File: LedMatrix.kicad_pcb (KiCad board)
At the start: 2 copper layers, 32 x 32 mm, 30 parts, among them IC1 ATMEGA328P-A, P1 FTDI, P2 SYNC_OUT, P3 ICSP, SW1 SW_PUSH, SW2 SWITCH_INV, U1 74HC238, U2 TD62083AFNG, U3 MCP1700-3302, U4 PNJ4K01F, U5 ADXL345, X1 8Mhz

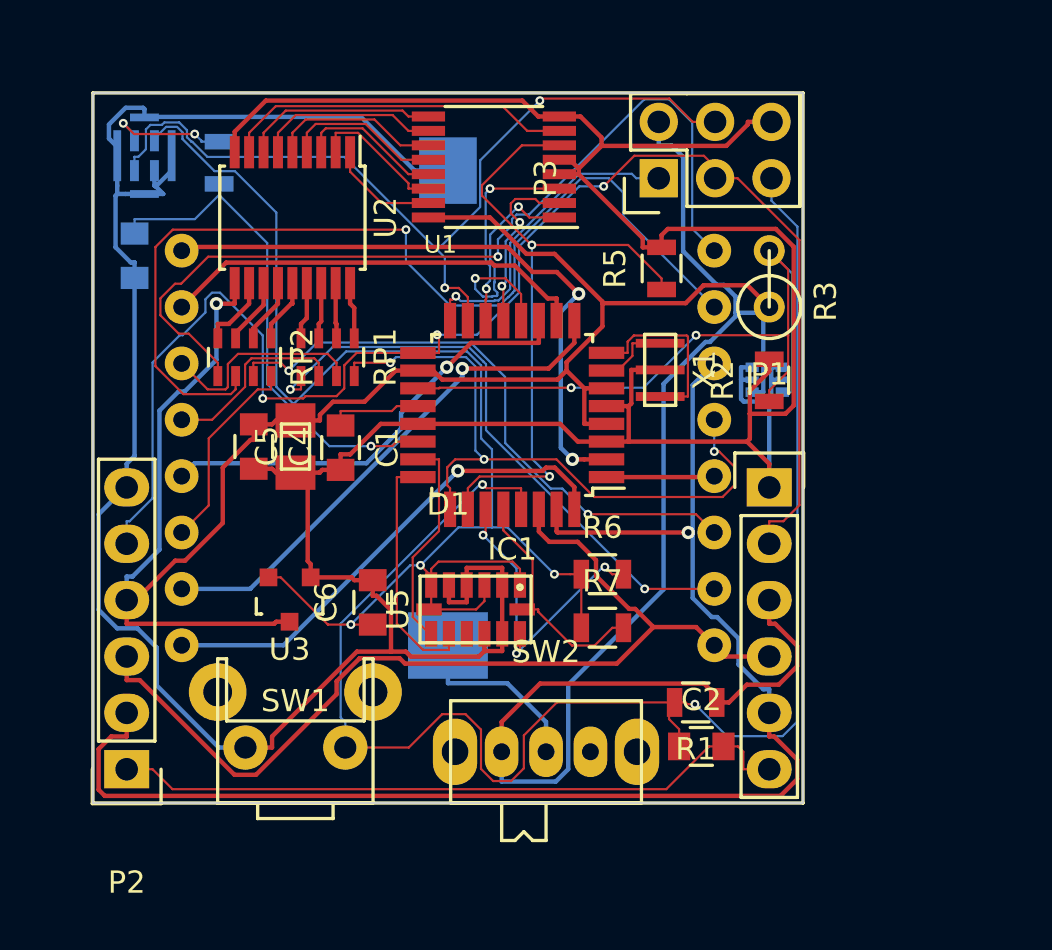
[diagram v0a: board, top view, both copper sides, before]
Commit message: Brightness code
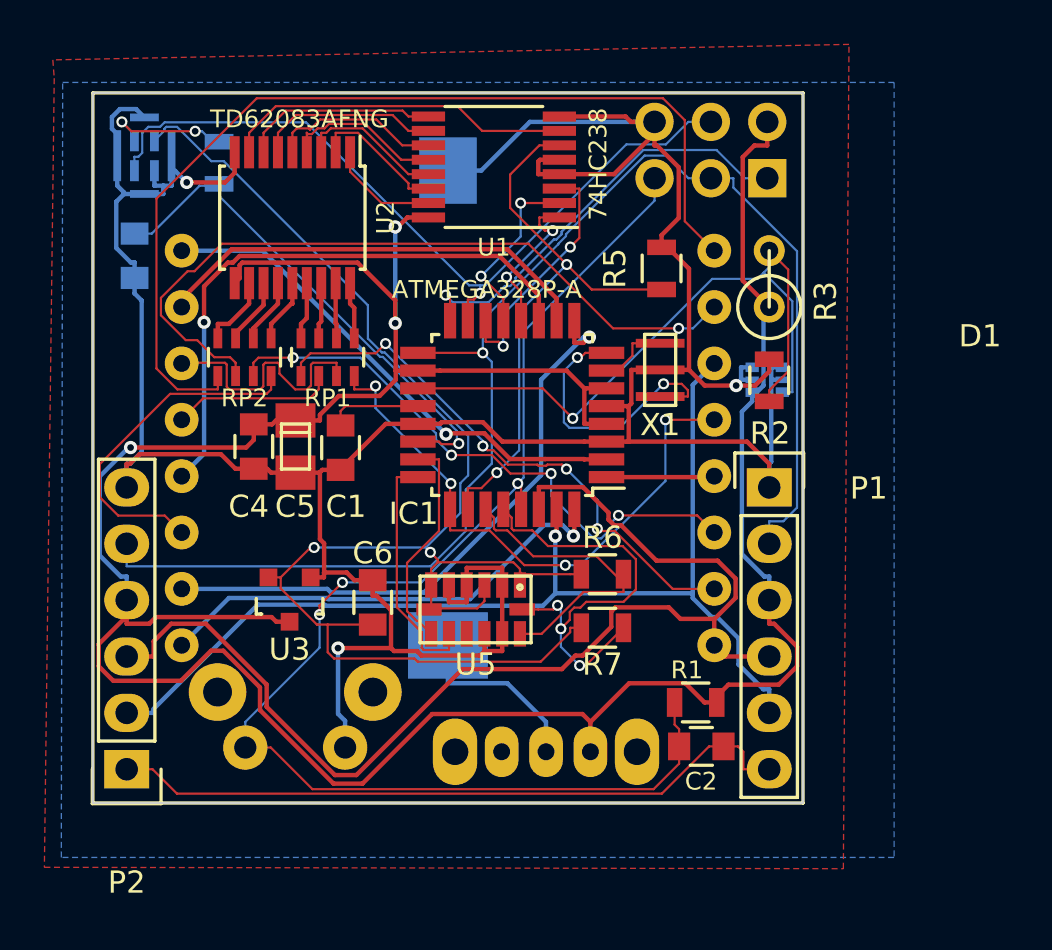
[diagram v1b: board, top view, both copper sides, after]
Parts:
- P3, SW1, SW2: moved to B.Cu
- moved P3 4.89 mm to (64.4, 37.8)
- turned SW1 to 180 degrees
- turned SW2 to 180 degrees
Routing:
- net GND: track 188.6 -> 149.9 mm, vias 0 -> 3
- net /ROW2: track 65.0 -> 49.6 mm
- net VCC: track 143.3 -> 132.1 mm, vias 1 -> 3
- net Net-(D1-Pad15): track 44.6 -> 33.6 mm
- net /RESET: track 71.1 -> 60.2 mm, vias 2 -> 3
- net /SCL: track 10.7 -> 20.4 mm, vias 0 -> 3
- net /ROW1: track 44.0 -> 52.5 mm
- net /ROW8: track 20.0 -> 26.5 mm
- net Net-(D1-Pad6): track 9.07 -> 15.5 mm
- net /ROW5: track 28.4 -> 23.1 mm, vias 2 -> 1
- net /MISO: track 14.2 -> 19.4 mm
- net Net-(IC1-Pad12): track 11.9 -> 7.14 mm
- net /LOWSIDE_EN: track 30.5 -> 25.8 mm
- net Net-(IC1-Pad8): track 8.26 -> 12.7 mm, vias 0 -> 2
- net Net-(D1-Pad16): track 39.8 -> 43.9 mm, vias 1 -> 0
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- added copper zone on B.Cu, net GND
- added copper zone on F.Cu, net GND
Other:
- net class SIGNAL: via_dia 0.4 -> 0.5; via_drill 0.2 -> 0.3
- board text added: "DotDotLab"
- board text added: "EdwardRF Mika Lin"

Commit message: Add francis and northy mods
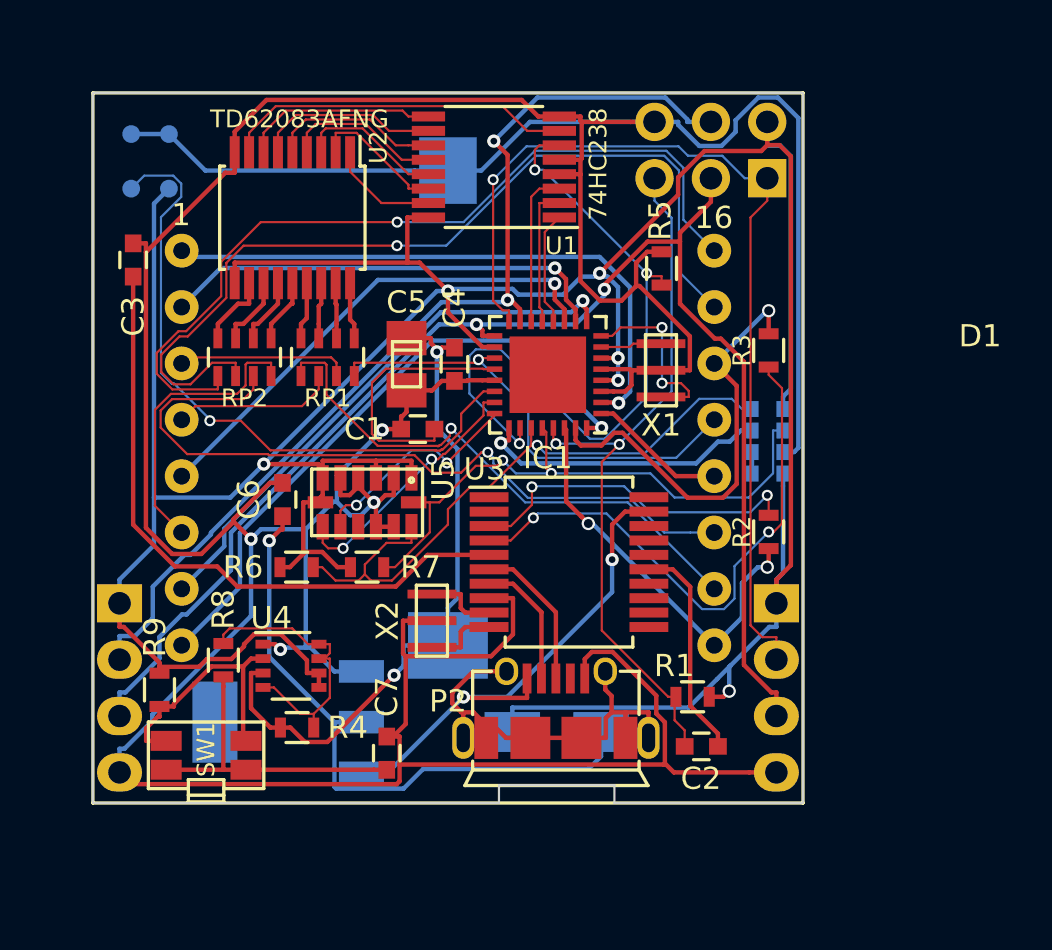
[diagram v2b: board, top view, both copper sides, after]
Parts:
- removed S1: MP34DT01, MP34DT01:MP34DT01
- removed SW2: SWITCH_INV, 1P2T:1P2T_SideSwitch
- added C7: 1uf, Capacitors_SMD:C_0603, F.Cu at (47.2, 63.8)
- added D2: D_Schottky, Diodes_SMD:SMA_Standard, B.Cu at (54.9, 62.8)
- added M1: 3729Mic, 3729Mic:3729Mic, B.Cu at (36.6, 37.1)
- added P0: CONN_01X04, Pin_Headers:Pin_Header_Straight_1x04, B.Cu at (64.8, 57.0)
- added R8: 100k, Resistors_SMD:R_0603, F.Cu at (39.9, 59.6)
- added R9: 10k, Resistors_SMD:R_0603, F.Cu at (37.0, 60.9)
- added U6: APDS-9900, ADPS-9900:ADPS-9900, B.Cu at (64.4, 49.7)
- added U7: AP1117D30, TO_SOT_Packages_SMD:SOT-223, B.Cu at (42.8, 62.4)
- added X2: 12Mhz, CSTCE8M:CSTCE8M00G52, F.Cu at (49.3, 57.8)
- C1, C2, C4, C6: footprint Capacitors_SMD:C_0805 -> Capacitors_SMD:C_0603
- C3: value 10nf -> 0.1uf; footprint Capacitors_SMD:C_0805 -> Capacitors_SMD:C_0603; moved to F.Cu
- IC1: footprint Housings_QFP:TQFP-32_7x7mm_Pitch0.8mm -> Housings_DFN_QFN:QFN-32-1EP_5x5mm_Pitch0.5mm
- P1: value FTDI -> CONN_01X04; footprint Pin_Headers:Pin_Header_Straight_1x06 -> Pin_Headers:Pin_Header_Straight_1x04; moved to B.Cu
- P2: value SYNC_OUT -> USB_OTG; footprint Pin_Headers:Pin_Header_Straight_1x06 -> Molex475890001:47589-0001
- R1, R2, R5, R6, R7: footprint Resistors_SMD:R_0805 -> Resistors_SMD:R_0603
- R3: value Photores -> 100k; footprint Discret:R1 -> Resistors_SMD:R_0603
- R4: footprint Resistors_SMD:R_0805 -> Resistors_SMD:R_0603; moved to F.Cu
- SW1: footprint SideButton:SidePushButton -> SKSCLCE010:SKSCLCE010; moved to F.Cu
- U3: value MCP1700-3302 -> CH340T; footprint Housings_SOT-23_SOT-143_TSOT-6:SOT-23 -> Housings_SSOP:SSOP-20_5.3x7.2mm_Pitch0.65mm
- U4: value PNJ4K01F -> TPCP8405; footprint pnj4k01f:KPTFTN6K0001 -> ps_8:PS-8; moved to F.Cu
- moved P1 29.7 mm to (35.2, 57.0), turned to 180 degrees
- moved R4 25.7 mm to (43.2, 62.6), turned to 0 degrees
- moved U4 25.0 mm to (42.9, 59.8)
- moved P2 19.4 mm to (54.9, 63.1), turned to 0 degrees
- moved R6 13.8 mm to (43.2, 55.4)
- moved U3 12.7 mm to (55.5, 55.1), turned to 0 degrees
- moved R7 11.0 mm to (46.4, 55.4)
- moved C4 9.77 mm to (50.3, 46.2)
- moved U5 6.87 mm to (46.4, 52.5)
- moved R2 6.83 mm to (64.5, 53.8)
- moved C5 6.23 mm to (48.1, 46.2)
- moved C6 6.16 mm to (42.5, 52.3)
- moved SW1 4.03 mm to (39.1, 63.9), turned to 0 degrees
- moved C1 3.58 mm to (48.6, 49.1), turned to 180 degrees
- moved R3 3.23 mm to (64.5, 45.6), turned to 270 degrees
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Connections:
- C2 pad 2: /DTR -> Net-(C2-Pad2)
- C3 pad 1: /AUDIO_IN -> GND
- C3 pad 2: GND -> Net-(C3-Pad2)
- C4 pad 1: VCC -> Net-(BT1-Pad1)
- C5 pad 1: VCC -> Net-(BT1-Pad1)
- C6 pad 1: /3v3 -> Net-(C6-Pad1)
- IC1 pad 15: /AUDIO_CLK -> /MOSI
- IC1 pad 17: /RTS -> /SCK
- IC1 pad 19: /LIGHT_SENSE -> /LED_SENSE
- IC1 pad 25: /LED_SENSE -> /LIGHT_INT
- P1 pad 1: GND -> VCC
- P1 pad 2: /RTS -> /MOSI
- P1 pad 3: VCC -> /SCK
- P1 pad 4: /ROW1 -> GND
- P2 pad 1: /DTR -> /5V
- P2 pad 2: /ROW2 -> /D-
- P2 pad 3: /ROW1 -> /D+
- P2 pad 4: VCC -> (no net)
- P2 pad 5: /RTS -> GND
- P2 pad 6: GND -> Net-(P2-Pad6)
- P3 pad 3: /RTS -> /SCK
- P3 pad 4: /AUDIO_CLK -> /MOSI
- R2 pad 1: /LIGHT_SENSE -> /ROW1
- R2 pad 2: GND -> Net-(R2-Pad2)
- R3 pad 1: VCC -> /ROW2
- R3 pad 2: /LIGHT_SENSE -> Net-(R3-Pad2)
- R4 pad 1: /AUDIO_IN -> Net-(BT1-Pad1)
- R6 pad 1: /3v3 -> VCC
- R7 pad 1: /3v3 -> VCC
- SW1 pad 1: GND -> Net-(C7-Pad1)
- SW1 pad 2: /RESET -> Net-(R9-Pad2)
- U3 pad 1: GND -> (no net)
- U3 pad 2: /3v3 -> (no net)
- U3 pad 3: VCC -> Net-(R2-Pad2)
- U4 pad 1: VCC -> GND
- U4 pad 2: GND -> Net-(R9-Pad2)
- U4 pad 3: GND -> Net-(BT1-Pad1)
- U4 pad 4: GND -> Net-(R4-Pad2)
- U4 pad 5: GND -> VCC
- U4 pad 6: /LIGHT_SENSE -> VCC
- U5 pad 1: /3v3 -> VCC
- U5 pad 3: /3v3 -> VCC
- U5 pad 6: /3v3 -> VCC
- U5 pad 7: /3v3 -> VCC
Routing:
- net GND: track 149.9 -> 228.7 mm, vias 3 -> 4
- net /3v3: track 67.3 -> 0.00 mm, vias 2 -> 0
- net /SCK: track 0.00 -> 64.7 mm, vias 0 -> 2
- net /RTS: track 63.4 -> 0.00 mm, vias 1 -> 0
- net /MOSI: track 0.00 -> 45.5 mm, vias 0 -> 2
- net VCC: track 132.1 -> 170.0 mm, vias 3 -> 6
- net /AUDIO_CLK: track 35.8 -> 0.00 mm, vias 1 -> 0
- net /ROW1: track 52.5 -> 18.3 mm, vias 0 -> 2
- net /LIGHT_SENSE: track 33.8 -> 0.00 mm, vias 1 -> 0
- net /DTR: track 31.2 -> 0.00 mm
- net /ROW2: track 49.6 -> 19.9 mm
- net Net-(C3-Pad2): track 0.00 -> 29.0 mm
- net Net-(C6-Pad1): track 0.00 -> 28.7 mm, vias 0 -> 1
- net /RESET: track 60.2 -> 32.4 mm, vias 3 -> 2
- net Net-(R3-Pad2): track 0.00 -> 25.2 mm, vias 0 -> 2
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- removed copper zone on B.Cu, net GND
- removed copper zone on F.Cu, net GND
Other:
- outline, holes or cut-outs redrawn
- board text added: "1"
- board text added: "16"
- board text added: "G"
- board text added: "Gnd"
- board text added: "ICSP"
- board text added: "Miso"
- board text added: "Mosi"
- board text added: "PWR"
- board text added: "Sck"
- board text added: "Vcc"
- board text added: "isobar"
- board text added: "nowlab"
- board text removed: "DotDotLab"
- board text removed: "EdwardRF Mika Lin"
